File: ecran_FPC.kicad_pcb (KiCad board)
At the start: 4 copper layers, 43 x 43 mm, 24 parts, among them J1 MEC1-110-02-F-D-A, J2 MEC1-110-02-F-D-A, J3 1-2328724-5, SW1 PEC11L-4220K-S0015

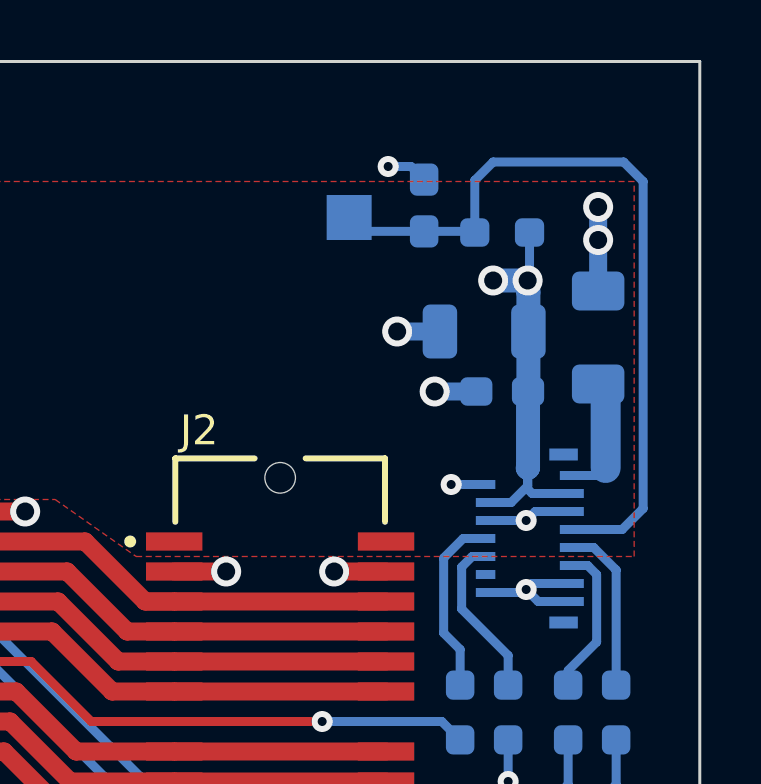
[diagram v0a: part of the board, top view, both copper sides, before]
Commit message: daily
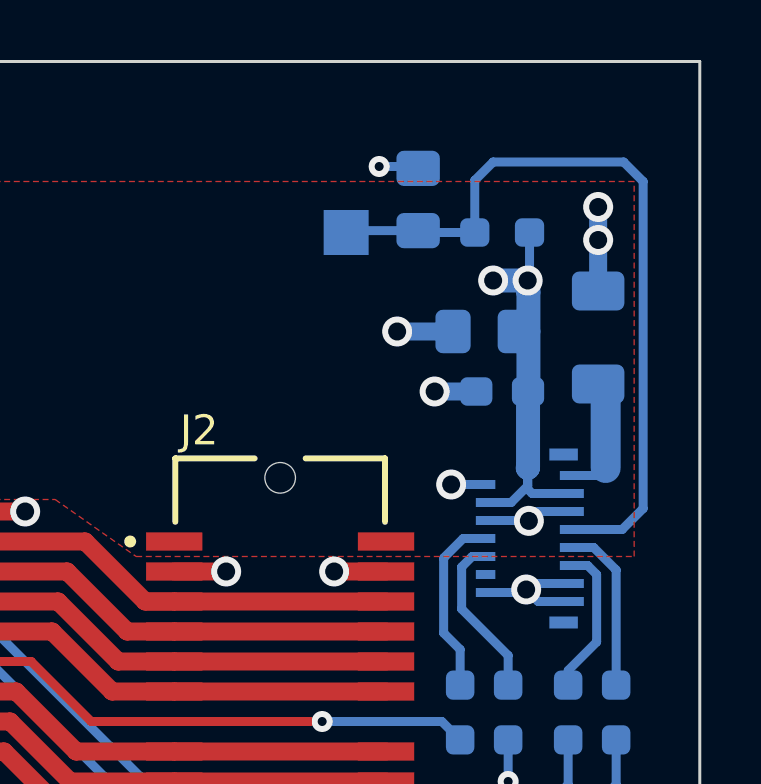
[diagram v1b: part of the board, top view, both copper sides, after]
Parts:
- C1: value 1µ -> 1µ 50V; footprint Capacitor_SMD:C_0603_1608Metric_Pad1.08x0.95mm_HandSolder -> Capacitor_SMD:C_0805_2012Metric_Pad1.18x1.45mm_HandSolder
- C2: value 4µ7 50V -> 4µ7 10V; footprint Capacitor_SMD:C_1206_3216Metric -> Capacitor_SMD:C_0805_2012Metric_Pad1.18x1.45mm_HandSolder
- C3: value 0.1µ -> 0.1µ 10V
- C4, C5: value 0.1u -> 0.1µ 10V
- C6: value 10n -> 0.1µ 10V
- moved TP1 0.51 mm to (131.2, 105.7)
- moved C1 0.28 mm to (133.6, 104.6)
